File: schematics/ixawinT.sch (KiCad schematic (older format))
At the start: 6 parts, among them U1 LM358

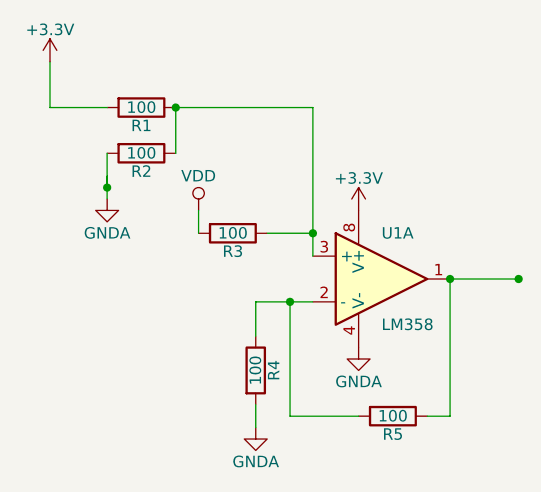
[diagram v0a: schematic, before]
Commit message: Added first iteration of the board
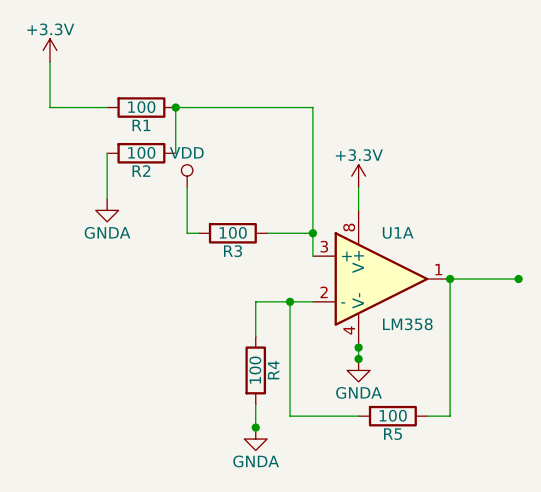
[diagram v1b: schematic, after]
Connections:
- wire segments 17 -> 19
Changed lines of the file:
@@
 LIBS:contrib
 LIBS:valves
+LIBS:ixawinT-cache
 EELAYER 25 0
 EELAYER END
@@
 $EndComp
 $Comp
-L +3.3V #PWR4
-U 1 1 5D13BD13
-P 2150 1850
-F 0 "#PWR4" H 2150 1700 50  0001 C CNN
-F 1 "+3.3V" H 2150 1990 50  0000 C CNN
-F 2 "" H 2150 1850 50  0000 C CNN
-F 3 "" H 2150 1850 50  0000 C CNN
-	1    2150 1850
-	1    0    0    -1
-$EndComp
-$Comp
-L GNDA #PWR2
+L GNDA #GND01
 U 1 1 5D13BD2D
 P 1050 1800
-F 0 "#PWR2" H 1050 1550 50  0001 C CNN
+F 0 "#GND01" H 1050 1550 50  0001 C CNN
 F 1 "GNDA" H 1050 1650 50  0000 C CNN
 F 2 "" H 1050 1800 50  0000 C CNN
@@
 $EndComp
 $Comp
-L +3.3V #PWR1
-U 1 1 5D13BE3A
-P 800 1200
-F 0 "#PWR1" H 800 1050 50  0001 C CNN
-F 1 "+3.3V" H 800 1340 50  0000 C CNN
-F 2 "" H 800 1200 50  0000 C CNN
-F 3 "" H 800 1200 50  0000 C CNN
-	1    800  1200
-	1    0    0    -1
-$EndComp
-$Comp
-L GNDA #PWR5
+L GNDA #PWR02
 U 1 1 5D13BE50
-P 2150 2450
-F 0 "#PWR5" H 2150 2200 50  0001 C CNN
-F 1 "GNDA" H 2150 2300 50  0000 C CNN
-F 2 "" H 2150 2450 50  0000 C CNN
-F 3 "" H 2150 2450 50  0000 C CNN
-	1    2150 2450
+P 2150 2500
+F 0 "#PWR02" H 2150 2250 50  0001 C CNN
+F 1 "GNDA" H 2150 2350 50  0000 C CNN
+F 2 "" H 2150 2500 50  0000 C CNN
+F 3 "" H 2150 2500 50  0000 C CNN
+	1    2150 2500
 	1    0    0    -1
 $EndComp
@@
 $EndComp
 Wire Wire Line
-	1050 1400 800  1400
-Wire Wire Line
-	800  1400 800  1200
-Wire Wire Line
 	1350 1400 1950 1400
 Wire Wire Line
@@
 Wire Wire Line
 	1350 1400 1350 1600
-Wire Wire Line
-	1050 1700 1050 1800
-Wire Wire Line
-	1050 1600 1050 1750
-Connection ~ 1050 1750
-$Comp
-L VDD #IN1
-U 1 1 5D13C4BE
-P 1450 1850
-F 0 "#IN1" H 1450 1700 50  0001 C CNN
-F 1 "VDD" H 1450 2000 50  0000 C CNN
-F 2 "" H 1450 1850 50  0000 C CNN
-F 3 "" H 1450 1850 50  0000 C CNN
-	1    1450 1850
-	1    0    0    -1
-$EndComp
 $Comp
 L R R3
@@
 $EndComp
 Wire Wire Line
-	1450 1950 1450 1850
-Wire Wire Line
 	1750 1950 1950 1950
 Connection ~ 1950 1950
 $Comp
-L GNDA #PWR3
+L GNDA #PWR03
 U 1 1 5D13C682
 P 1700 2800
-F 0 "#PWR3" H 1700 2550 50  0001 C CNN
+F 0 "#PWR03" H 1700 2550 50  0001 C CNN
 F 1 "GNDA" H 1700 2650 50  0000 C CNN
 F 2 "" H 1700 2800 50  0000 C CNN
@@
 $EndComp
 Wire Wire Line
-	1950 2250 1700 2250
+	1700 2250 1950 2250
 $Comp
 L R R5
@@
 Connection ~ 1350 1400
 Connection ~ 2550 2150
+Wire Wire Line
+	2150 2450 2150 2500
+Connection ~ 1700 2800
+Connection ~ 2150 2450
+Connection ~ 2150 2500
+Wire Wire Line
+	800  1200 800  1400
+Wire Wire Line
+	800  1400 1050 1400
+Wire Wire Line
+	2150 1750 2150 1850
+Wire Wire Line
+	1050 1600 1050 1800
+$Comp
+L +3.3V #PWR04
+U 1 1 5D150409
+P 800 1200
+F 0 "#PWR04" H 800 1050 50  0001 C CNN
+F 1 "+3.3V" H 800 1340 50  0000 C CNN
+F 2 "" H 800 1200 50  0000 C CNN
+F 3 "" H 800 1200 50  0000 C CNN
+	1    800  1200
+	1    0    0    -1
+$EndComp
+$Comp
+L +3.3V #PWR05
+U 1 1 5D150469
+P 2150 1750
+F 0 "#PWR05" H 2150 1600 50  0001 C CNN
+F 1 "+3.3V" H 2150 1890 50  0000 C CNN
+F 2 "" H 2150 1750 50  0000 C CNN
+F 3 "" H 2150 1750 50  0000 C CNN
+	1    2150 1750
+	1    0    0    -1
+$EndComp
+$Comp
+L VDD #IN06
+U 1 1 5D1504A8
+P 1400 1750
+F 0 "#IN06" H 1400 1600 50  0001 C CNN
+F 1 "VDD" H 1400 1900 50  0000 C CNN
+F 2 "" H 1400 1750 50  0000 C CNN
+F 3 "" H 1400 1750 50  0000 C CNN
+	1    1400 1750
+	1    0    0    -1
+$EndComp
+Wire Wire Line
+	1450 1950 1400 1950
+Wire Wire Line
+	1400 1950 1400 1750
 $EndSCHEMATC
